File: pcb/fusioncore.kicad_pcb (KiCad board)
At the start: 2 copper layers, 95 x 99 mm, 107 parts, among them J1 Conn_02x12_Top_Bottom, J10 Pump_Misc_1, J11 Pump_Misc_2, J12 Flow_Warm, J13 Flow_Cold, J14 Trigger, J15 Valve_M1, J16 Valve_M2, J17 Valve_M3, J18 Valve_M4, J19 Valve_Air_Lime, J2 Temp_1, J20 Valve_Air_Rum, J21 Valve_Air_Out, J22 LED, J3 40HAT, J4 Temp_2, J5 WEIGHT, J6 Pump_Water_Cold, J7 Pump_Water_Warm, J8 Pump_Air, J9 CONN_01X02, Q1 DMG2305UX, Q10 AO3400A, Q11 AO3400A, Q12 AO3400A, Q13 AO3400A, Q14 AO3400A, Q15 BSS138, Q16 S8550, Q17 AO3400A, Q18 AO3400A, Q2 DMMT5401, Q3 AO3400A, Q4 AO3400A, Q5 AO3400A, Q6 AO3400A, Q7 AO3400A, Q8 AO3400A, Q9 AO3400A, U1 HX711, U2 CAT24C32, U3 LTC2990, U4 LTC2990

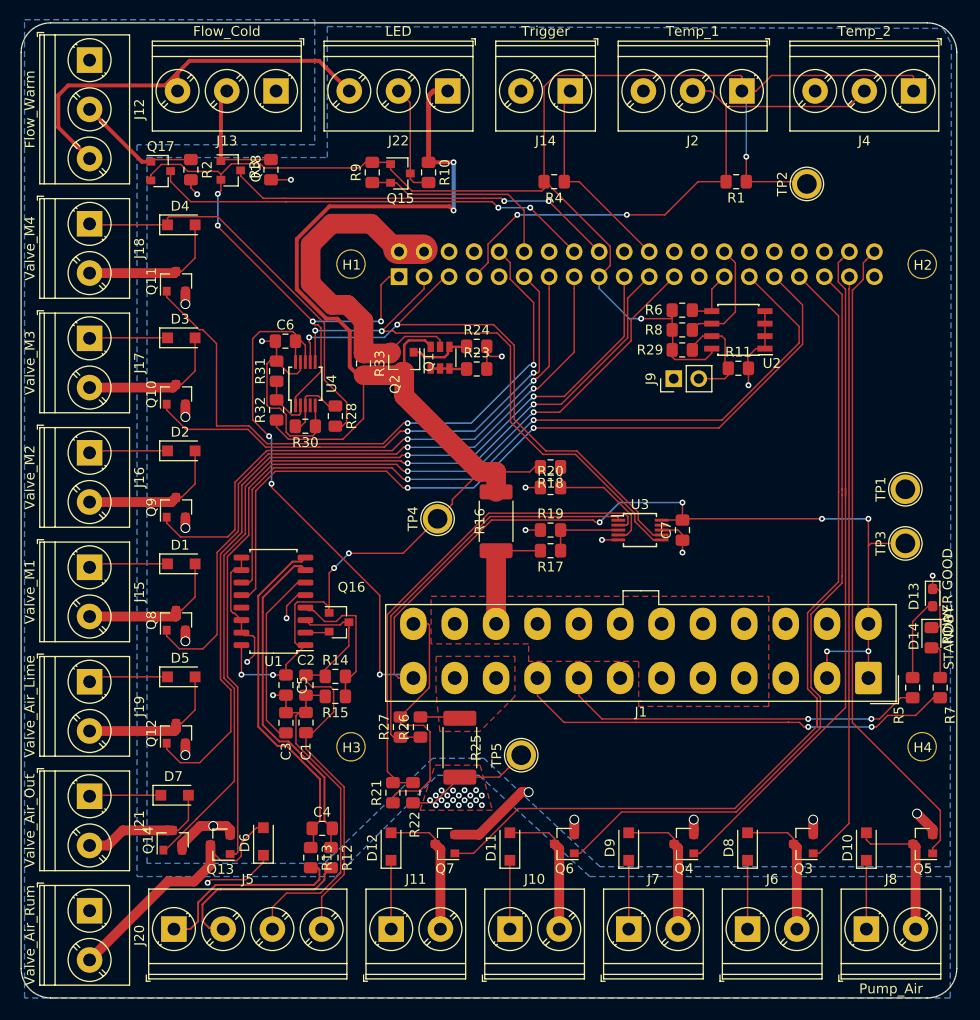
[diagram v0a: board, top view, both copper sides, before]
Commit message: Minor PCB fixes.
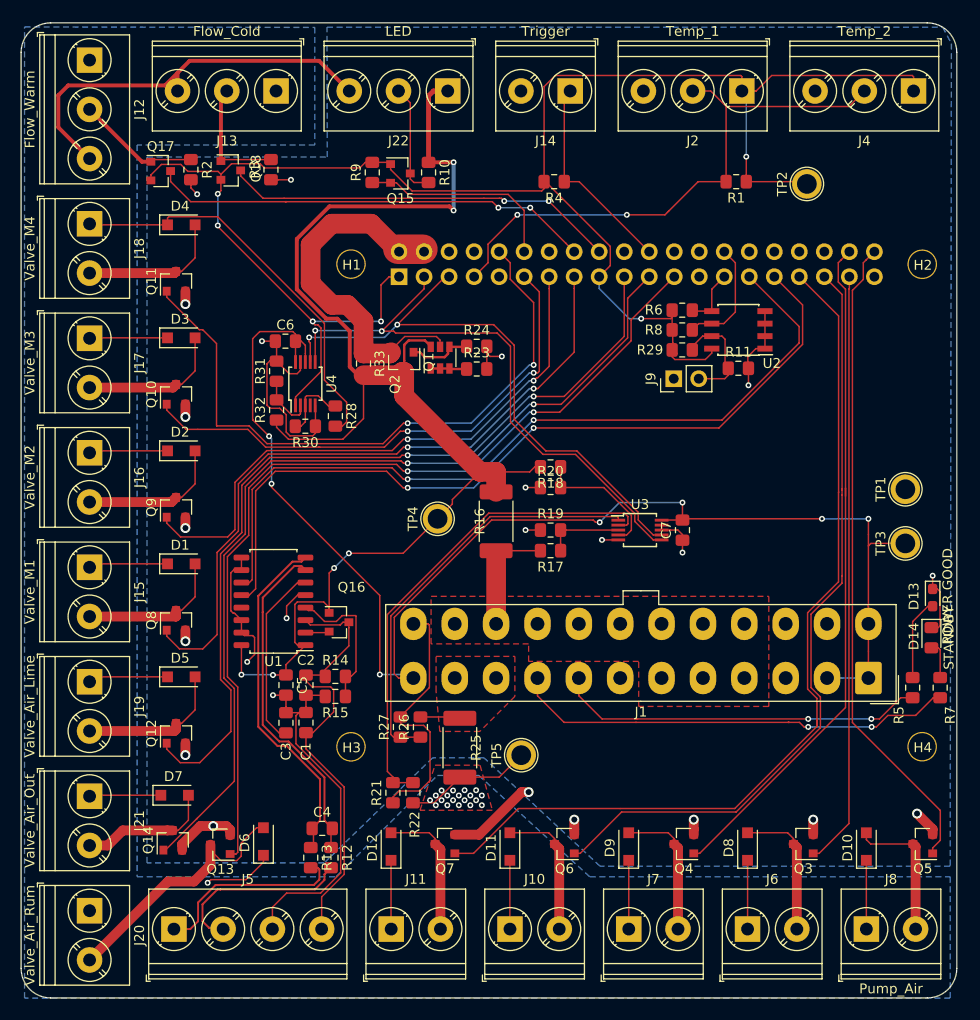
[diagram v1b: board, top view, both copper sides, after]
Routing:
- net /3V3: track 145.4 -> 142.7 mm, vias 9 -> 7
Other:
- rule pad_to_mask_clearance: 0.1 -> 0.08
